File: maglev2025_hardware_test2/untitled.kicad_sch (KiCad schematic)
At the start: 37 parts, among them J3 Conn_01x04, J4 Conn_01x04_MountingPin, J5 USB_C_Receptacle_USB2.0, J6 Conn_01x04, SW4 RotaryEncoder_Switch_MP

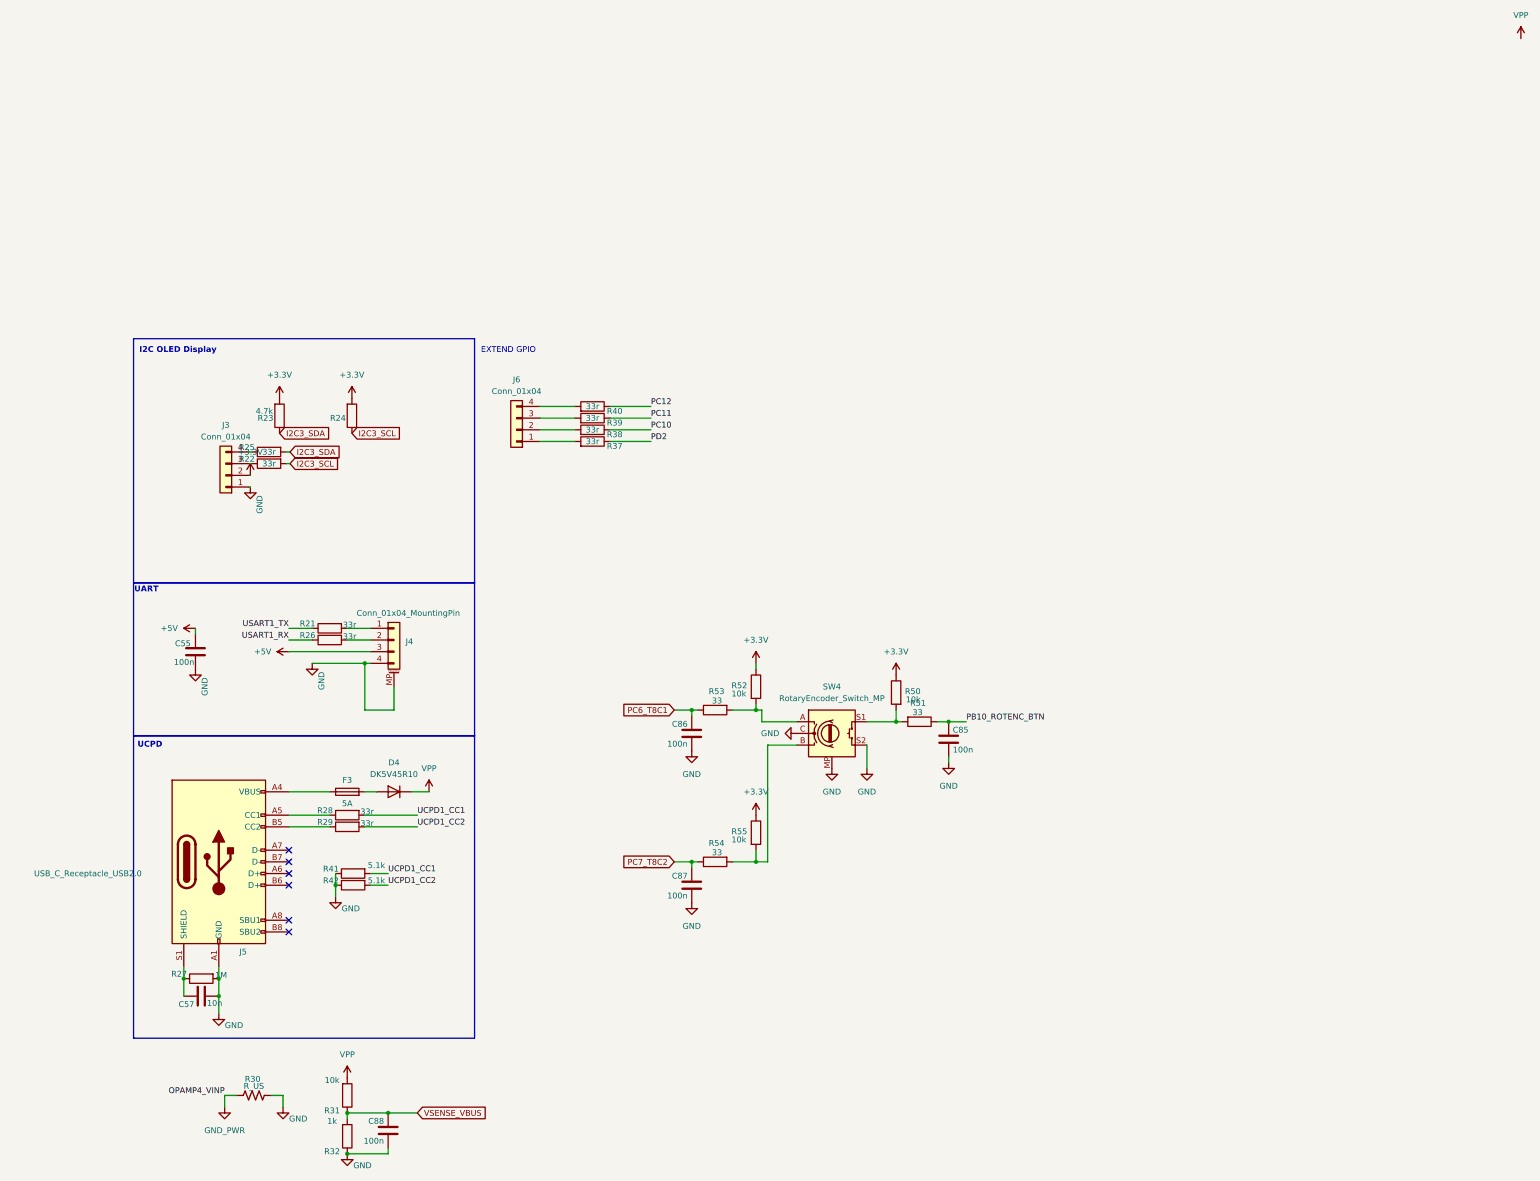
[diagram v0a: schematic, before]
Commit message: addjust layout
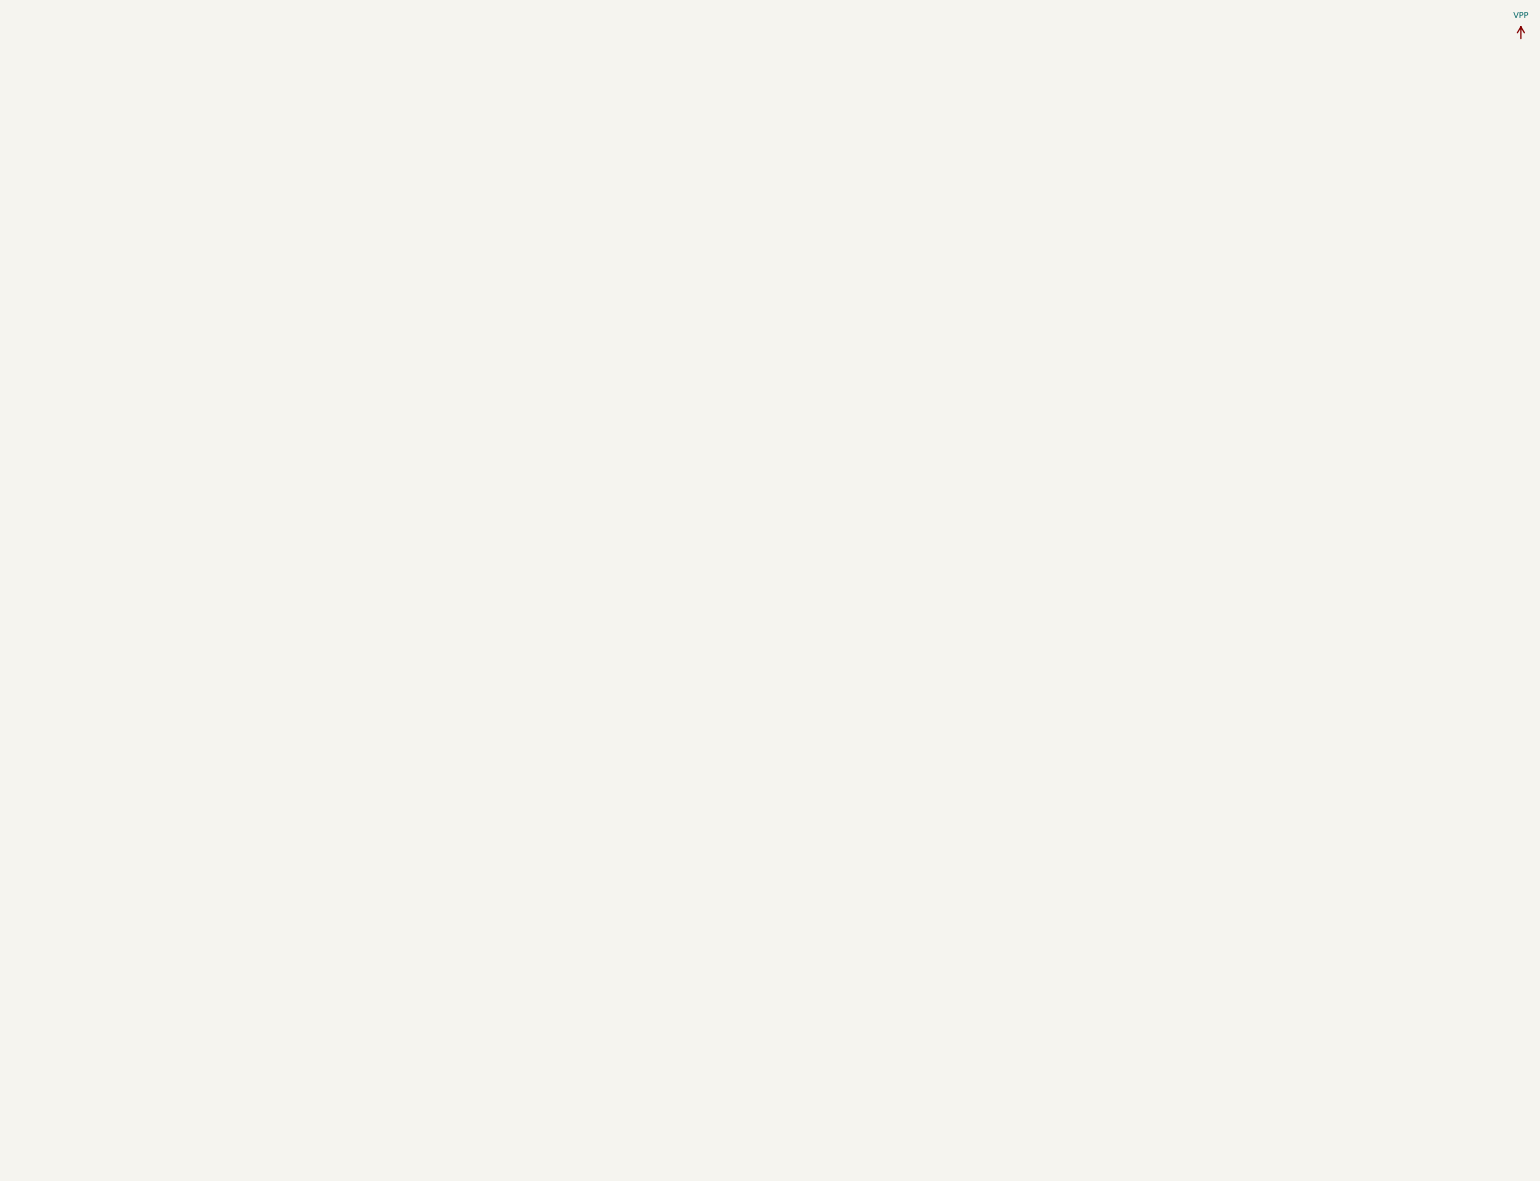
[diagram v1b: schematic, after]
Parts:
- removed C55, C85, C86, C87, C88: 100n, Capacitor_SMD:C_0603_1608Metric, symbol Device:C
- removed C57: 10n, Capacitor_SMD:C_0603_1608Metric, symbol Device:C
- removed D4: DK5V45R10, Diode_SMD:D_PowerDI-5, symbol Device:D
- removed F3: 5A, Fuse:Fuse_1206_3216Metric, symbol Device:Fuse
- removed J3, J6: Conn_01x04, Connector_PinHeader_2.54mm:PinHeader_1x04_P2.54mm_Vertical, symbol Connector_Generic:Conn_01x04
- removed J4: Conn_01x04_MountingPin, Connector_JST:JST_GH_BM04B-GHS-TBT_1x04-1MP_P1.25mm_Vertical, symbol Connector_Generic_MountingPin:Conn_01x04_MountingPin
- removed J5: USB_C_Receptacle_USB2.0, Connector_USB:USB_C_Receptacle_HRO_TYPE-C-31-M-12, symbol Connector:USB_C_Receptacle_USB2.0
- removed R21, R22, R25, R26, R28, R29, R37, R38, R39, R40: 33r, Resistor_SMD:R_0603_1608Metric, symbol Device:R
- removed R23, R24: 4.7k, Resistor_SMD:R_0603_1608Metric, symbol Device:R
- removed R27: 1M, Resistor_SMD:R_0603_1608Metric, symbol Device:R
- removed R30: R_US, Resistor_SMD:R_2512_6332Metric, symbol Device:R_US
- removed R31, R50, R52, R55: 10k, Resistor_SMD:R_0603_1608Metric, symbol Device:R
- removed R32: 1k, Resistor_SMD:R_0603_1608Metric, symbol Device:R
- removed R41, R42: 5.1k, Resistor_SMD:R_0603_1608Metric, symbol Device:R
- removed R51, R53, R54: 33, Resistor_SMD:R_0603_1608Metric, symbol Device:R
- removed SW4: RotaryEncoder_Switch_MP, Rotary_Encoder:RotaryEncoder_Alps_EC11E-Switch_Vertical_H20mm_MountingHoles, symbol Device:RotaryEncoder_Switch_MP
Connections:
- no-connect marks 6 -> 0
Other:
- note removed: "EXTEND GPIO"
- note removed: "I2C OLED Display"
- note removed: "UART"
- note removed: "UCPD"
